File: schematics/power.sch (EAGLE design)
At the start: 5 parts, among them X1 MINI-USB-32005-301, X2 6ESRM-P

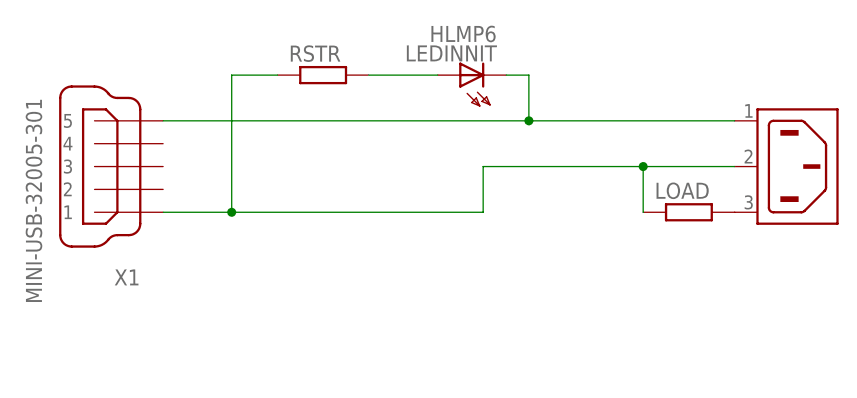
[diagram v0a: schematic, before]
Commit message: Updated schematic to latest version.
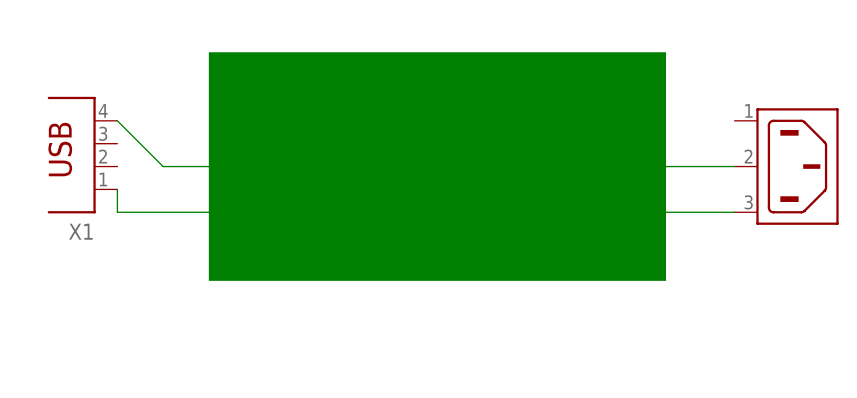
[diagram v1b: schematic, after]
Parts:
- removed LEDINNIT: HLMP6, display-hp:HLMP6
- removed LOAD, RSTR: (no value), rcl:R-EU_0207/10
- X1: value MINI-USB-32005-301 -> (none); device con-cypressindustries:MINI-USB-32005-301 -> con-berg:PN87520
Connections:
- removed net N$3: LEDINNIT.A, RSTR.2
- removed net N$4: LOAD.2, X2.AC2
- net N$1: now also X1.4; no longer LOAD.1, RSTR.1, X1.1
- net N$2: now also X1.1, X2.AC2; no longer LEDINNIT.K, X1.5, X2.AC1
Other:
- note added: "LIMITED CONFIDENTIAL"
- note added: "SLUGS TECH CORPORATION"
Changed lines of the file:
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@@
 </classes>
 <parts>
-<part name="X1" library="con-cypressindustries" deviceset="MINI-USB-" device="32005-301"/>
 <part name="X2" library="con-tycoelectronics" deviceset="6ESRM-P" device=""/>
-<part name="RSTR" library="rcl" deviceset="R-EU_" device="0207/10"/>
-<part name="LEDINNIT" library="display-hp" deviceset="HLMP6" device=""/>
-<part name="LOAD" library="rcl" deviceset="R-EU_" device="0207/10"/>
+<part name="X1" library="con-berg" deviceset="PN87520" device=""/>
 </parts>
 <sheets>
 <sheet>
 <plain>
+<rectangle x1="35.56" y1="33.02" x2="86.36" y2="58.42" layer="91"/>
+<text x="45.72" y="48.26" size="1.778" layer="94">SLUGS TECH CORPORATION</text>
+<text x="48.26" y="43.18" size="1.778" layer="94">LIMITED CONFIDENTIAL</text>
 </plain>
 <instances>
-<instance part="X1" gate="G$1" x="25.4" y="45.72" rot="R180"/>
 <instance part="X2" gate="G$1" x="96.52" y="45.72"/>
-<instance part="RSTR" gate="G$1" x="48.26" y="55.88"/>
-<instance part="LEDINNIT" gate="A" x="66.04" y="55.88" rot="R90"/>
-<instance part="LOAD" gate="G$1" x="88.9" y="40.64"/>
+<instance part="X1" gate="G$1" x="22.86" y="48.26" rot="R180"/>
 </instances>
 <busses>
@@
 <net name="N$1" class="0">
 <segment>
-<pinref part="X1" gate="G$1" pin="1"/>
-<wire x1="30.48" y1="40.64" x2="38.1" y2="40.64" width="0.1524" layer="91"/>
-<wire x1="38.1" y1="40.64" x2="66.04" y2="40.64" width="0.1524" layer="91"/>
-<wire x1="66.04" y1="40.64" x2="66.04" y2="45.72" width="0.1524" layer="91"/>
+<pinref part="X1" gate="G$1" pin="4"/>
 <pinref part="X2" gate="G$1" pin="SH"/>
-<wire x1="66.04" y1="45.72" x2="83.82" y2="45.72" width="0.1524" layer="91"/>
-<wire x1="83.82" y1="45.72" x2="93.98" y2="45.72" width="0.1524" layer="91"/>
-<wire x1="38.1" y1="40.64" x2="38.1" y2="55.88" width="0.1524" layer="91"/>
-<pinref part="RSTR" gate="G$1" pin="1"/>
-<wire x1="38.1" y1="55.88" x2="43.18" y2="55.88" width="0.1524" layer="91"/>
-<junction x="38.1" y="40.64"/>
-<pinref part="LOAD" gate="G$1" pin="1"/>
-<wire x1="83.82" y1="40.64" x2="83.82" y2="45.72" width="0.1524" layer="91"/>
-<junction x="83.82" y="45.72"/>
+<wire x1="25.4" y1="50.8" x2="30.48" y2="45.72" width="0.1524" layer="91"/>
+<wire x1="30.48" y1="45.72" x2="93.98" y2="45.72" width="0.1524" layer="91"/>
 </segment>
 </net>
 <net name="N$2" class="0">
 <segment>
-<pinref part="X1" gate="G$1" pin="5"/>
-<pinref part="X2" gate="G$1" pin="AC1"/>
-<wire x1="30.48" y1="50.8" x2="71.12" y2="50.8" width="0.1524" layer="91"/>
-<pinref part="LEDINNIT" gate="A" pin="K"/>
-<wire x1="71.12" y1="50.8" x2="93.98" y2="50.8" width="0.1524" layer="91"/>
-<wire x1="68.58" y1="55.88" x2="71.12" y2="55.88" width="0.1524" layer="91"/>
-<wire x1="71.12" y1="55.88" x2="71.12" y2="50.8" width="0.1524" layer="91"/>
-<junction x="71.12" y="50.8"/>
+<pinref part="X1" gate="G$1" pin="1"/>
+<pinref part="X2" gate="G$1" pin="AC2"/>
+<wire x1="25.4" y1="43.18" x2="25.4" y2="40.64" width="0.1524" layer="91"/>
+<wire x1="25.4" y1="40.64" x2="93.98" y2="40.64" width="0.1524" layer="91"/>
 </segment>
 </net>
-<net name="N$3" class="0">
-<segment>
-<pinref part="RSTR" gate="G$1" pin="2"/>
-<pinref part="LEDINNIT" gate="A" pin="A"/>
-<wire x1="53.34" y1="55.88" x2="60.96" y2="55.88" width="0.1524" layer="91"/>
-</segment>
-</net>
-<net name="N$4" class="0">
-<segment>
-<pinref part="X2" gate="G$1" pin="AC2"/>
-<pinref part="LOAD" gate="G$1" pin="2"/>
-</segment>
-</net>
